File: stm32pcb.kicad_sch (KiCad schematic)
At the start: 11 parts, among them J1 USB_C_Receptacle_USB2.0_16P, J2 Conn_01x04_Pin, J3 USB_C_Receptacle_USB2.0_16P, SW2 SW_Push_DPDT, U1 STM32F103C_8-B_Tx, U2 CH340C, U3 AMS1117-3.3

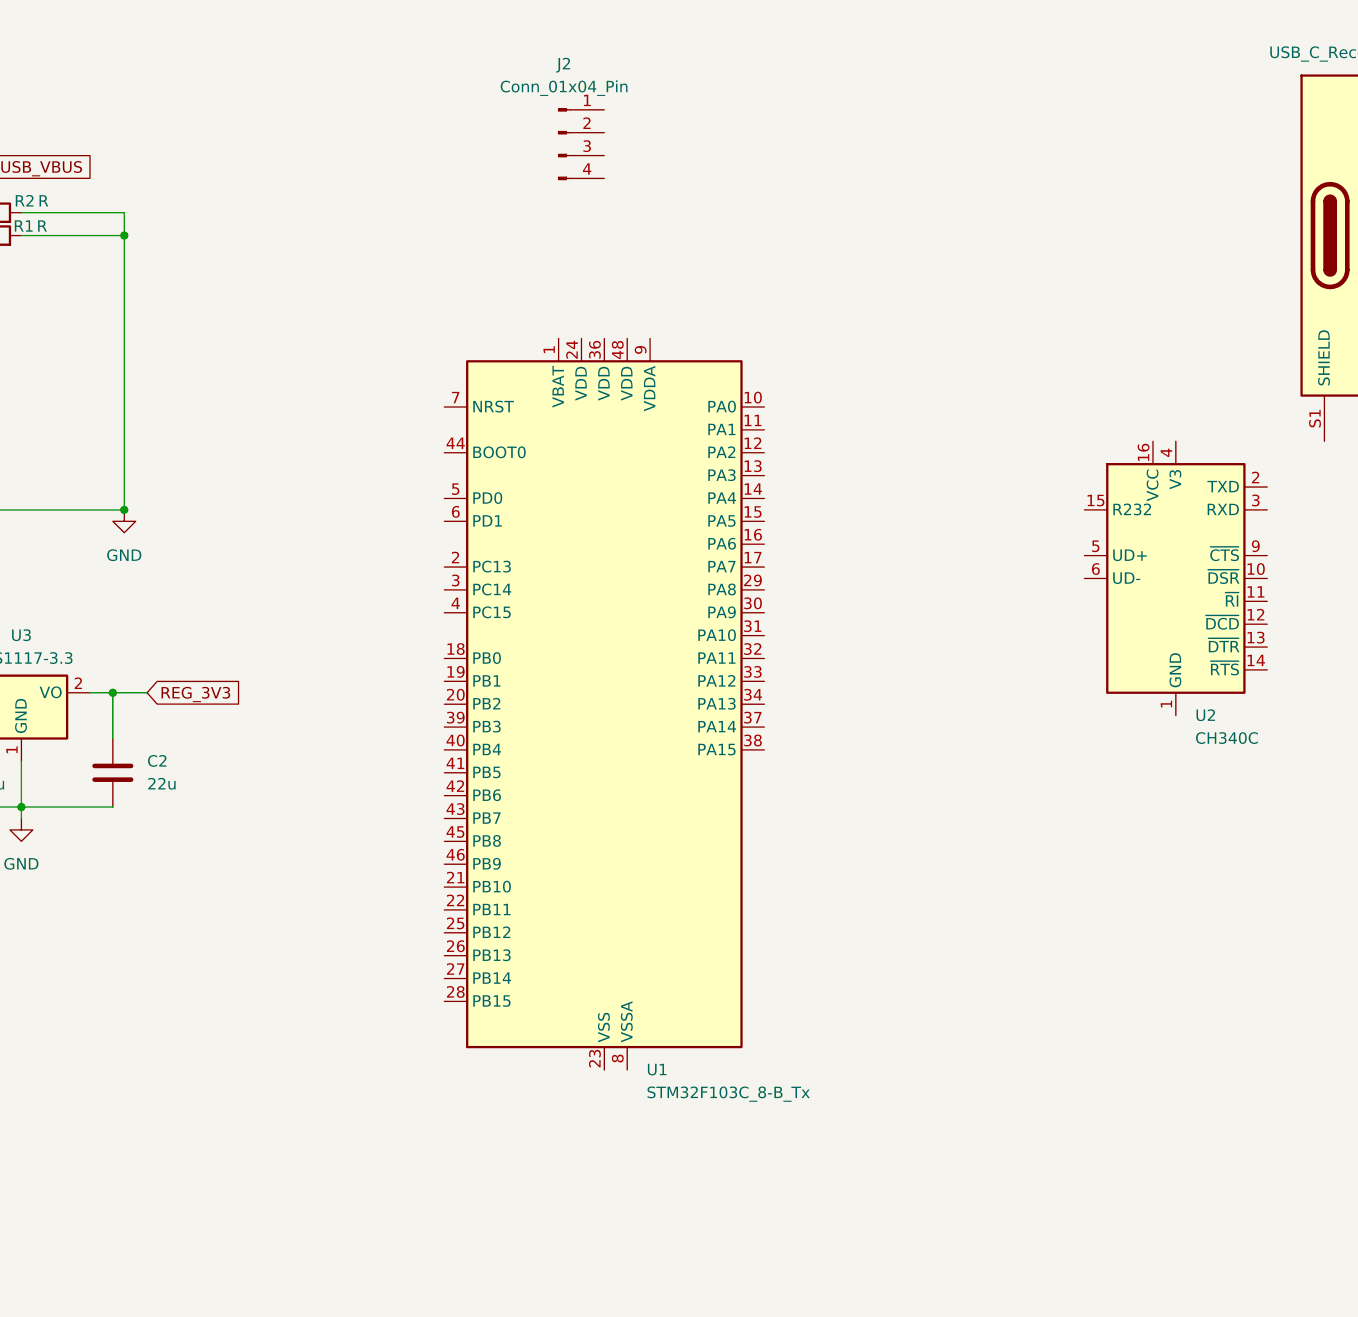
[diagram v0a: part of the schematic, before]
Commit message: 2
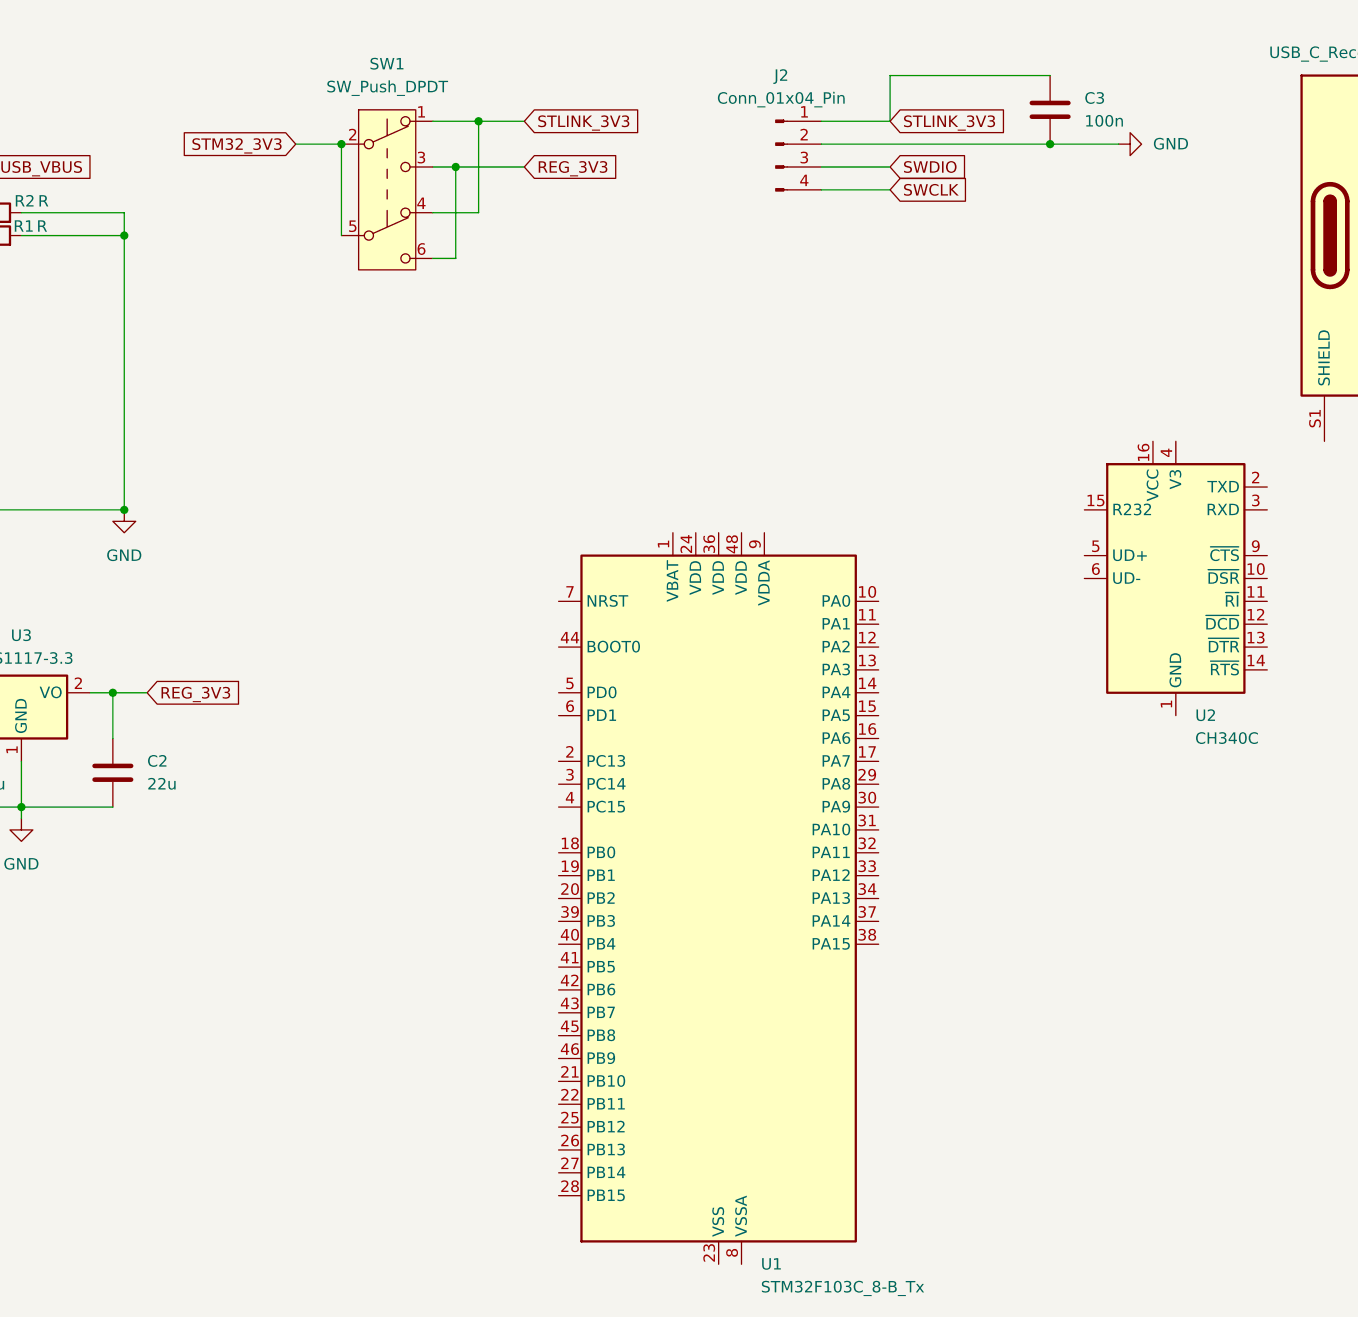
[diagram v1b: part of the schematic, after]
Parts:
- added C3: 100n, Capacitor_SMD:C_0805_2012Metric, symbol Device:C
- added SW1: SW_Push_DPDT, Button_Switch_SMD:SW_DPDT_CK_JS202011JCQN, symbol Switch:SW_Push_DPDT
- C1, C2: footprint (none) -> Capacitor_SMD:C_0805_2012Metric
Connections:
- net GND: now also J2.2 (Pin_2), C3.2
- net REG_3V3: now also SW1.3 (C), SW1.6 (C)
- net STLINK_3V3: now reaches J2.1 (Pin_1)
- net STLINK_3V3: now also C3.1, SW1.1 (A), SW1.4 (A)
- net SWDIO: now reaches J2.3 (Pin_3)
- net SWCLK: now reaches J2.4 (Pin_4)
- new net STM32_3V3: SW1.2 (B), SW1.5 (B)
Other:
- moved on the sheet: J2, U1

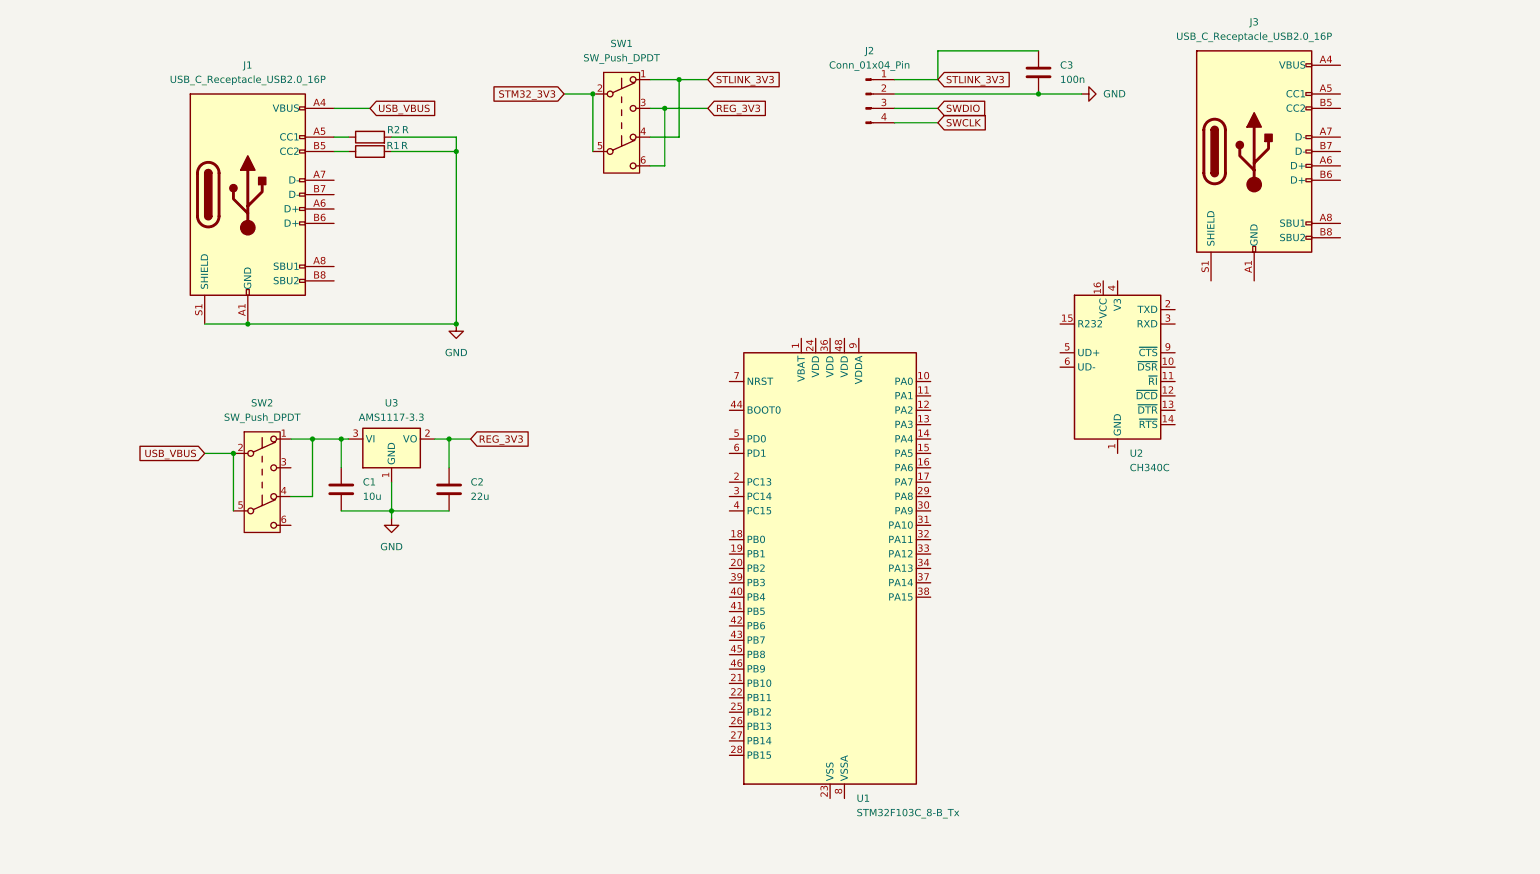
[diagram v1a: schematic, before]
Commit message: update
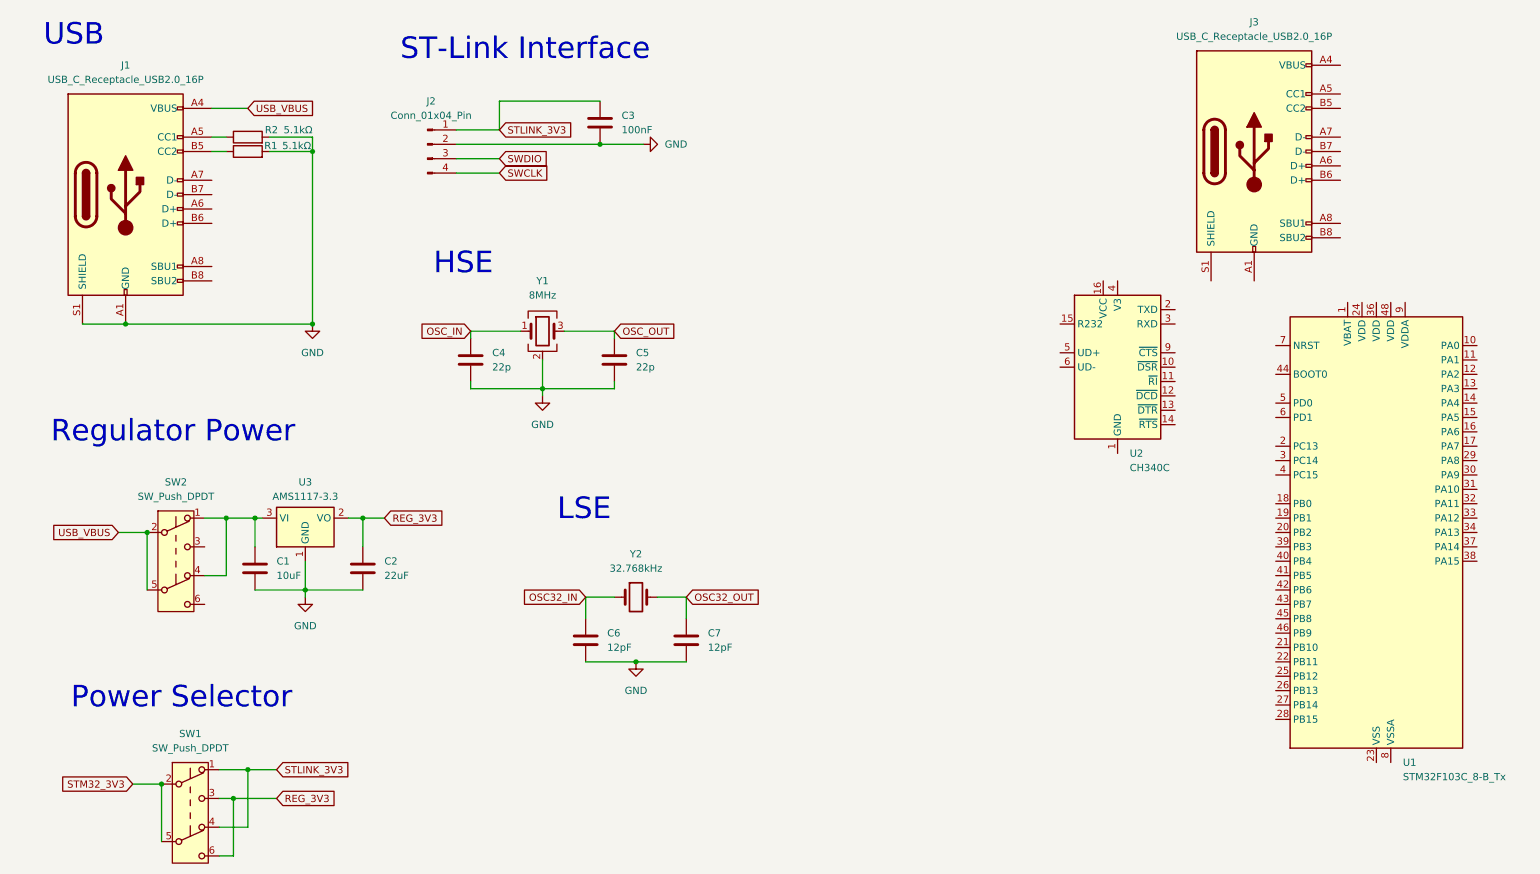
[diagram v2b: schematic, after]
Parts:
- added C4, C5: 22p, Capacitor_SMD:C_0805_2012Metric, symbol Device:C
- added C6, C7: 12pF, Capacitor_SMD:C_0805_2012Metric, symbol Device:C
- added Y1: 8MHz, symbol Device:Crystal_GND24
- added Y2: 32.768kHz, symbol Device:Crystal
- C1: value 10u -> 10uF
- C2: value 22u -> 22uF
- C3: value 100n -> 100nF
- R1, R2: value R -> 5.1kΩ
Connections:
- net GND: now also C4.2, C5.2, C6.2, C7.2, Y1.2 (G), Y1.4 (G)
- new net OSC32_IN: C6.1, Y2.1
- new net OSC32_OUT: C7.1, Y2.2
- new net OSC_IN: C4.1, Y1.1
- new net OSC_OUT: C5.1, Y1.3
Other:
- note added: "HSE"
- note added: "LSE"
- note added: "Power Selector"
- note added: "Regulator Power"
- note added: "ST-Link Interface"
- note added: "USB"
- moved on the sheet: C1, C2, C3, J1, J2, R1, R2, SW1, SW2, U1, U3

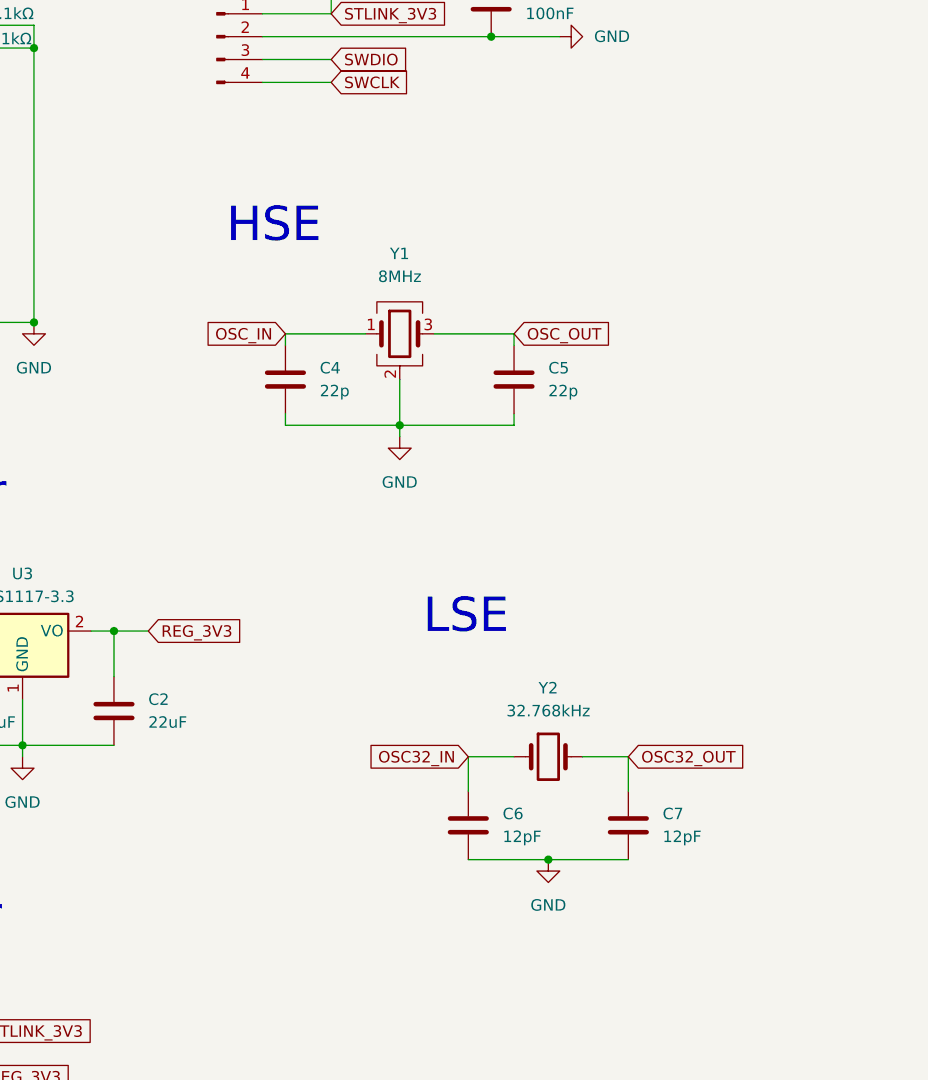
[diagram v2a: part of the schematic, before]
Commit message: update
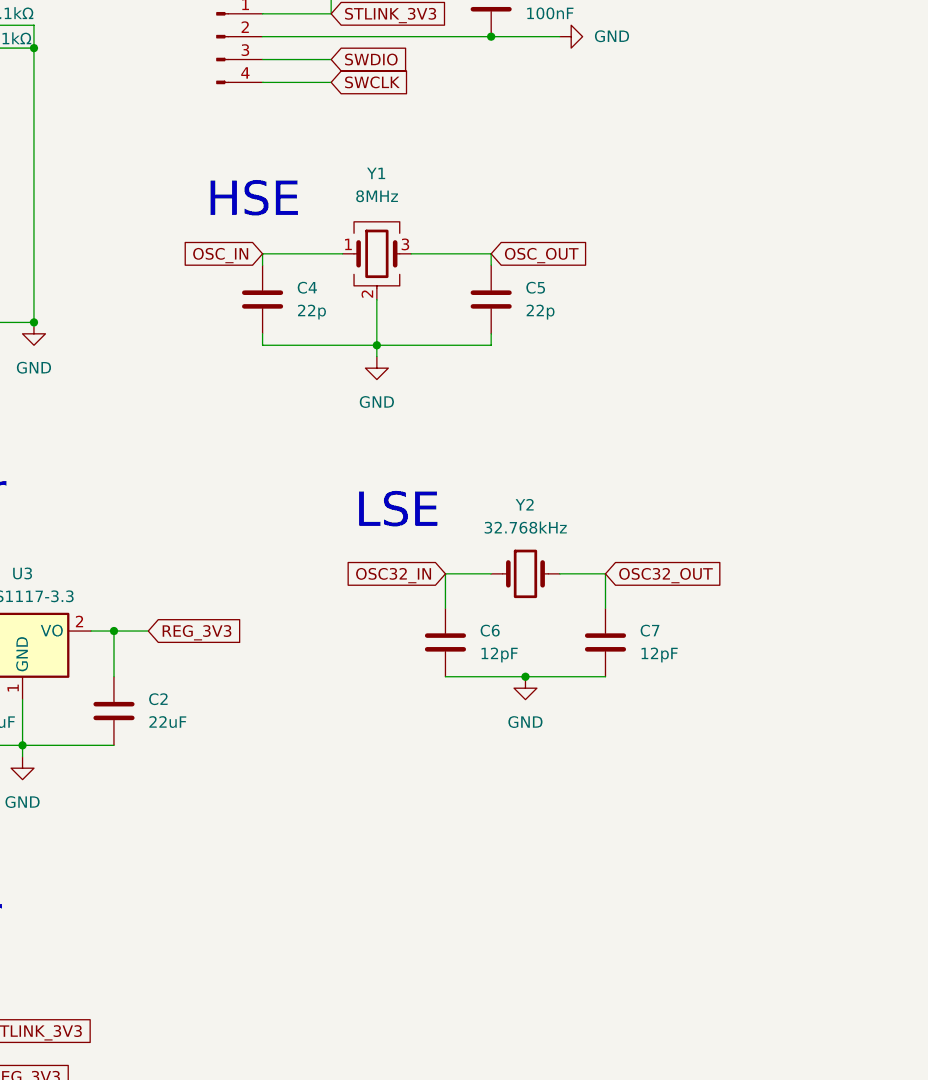
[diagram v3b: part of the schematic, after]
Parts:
- SW1: footprint Button_Switch_SMD:SW_DPDT_CK_JS202011JCQN -> lcsc:SW-SMD_6P-L9.1-W3.5-P2.50
- Y1: footprint (none) -> Crystal:Crystal_SMD_3225-4Pin_3.2x2.5mm
- Y2: footprint (none) -> Crystal:Crystal_SMD_3215-2Pin_3.2x1.5mm
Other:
- moved on the sheet: C4, C5, C6, C7, Y1, Y2

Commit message: update
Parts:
- added C10, C11, C12, C8, C9: 100nF, Capacitor_SMD:C_0805_2012Metric, symbol Device:C
- added D1, D2: LED, symbol Device:LED
- added J4: Conn_01x12_Pin, symbol Connector:Conn_01x12_Pin
- added R3, R4, R7: 10kΩ, Resistor_SMD:R_1206_3216Metric, symbol Device:R
- added R5, R6: 1kΩ, Resistor_SMD:R_1206_3216Metric, symbol Device:R
- added R8: 1.5kΩ, Resistor_SMD:R_1206_3216Metric, symbol Device:R
- added SW3, SW4: SW_Push_DPDT, Button_Switch_SMD:SW_DPDT_CK_JS202011JCQN, symbol Switch:SW_Push_DPDT
- added SW5: TS-1088-AR02016, lcsc:SW-SMD_L3.9-W3.0-P4.45, symbol lcsc:TS-1088-AR02016
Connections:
- net GND: now also U1.23 (VSS), U1.35 (VSS), U1.47 (VSS), U1.8 (VSSA), C10.2, C11.2, C12.2, C8.2, C9.2, D1.1 (K), D2.1 (K), J4.8 (Pin_8), SW3.3 (C), SW3.6 (C), SW4.3 (C), SW4.6 (C), SW5.1
- net REG_3V3: now also R5.2
- net STLINK_3V3: now also R6.2
- net STM32_3V3: now also U1.24 (VDD), U1.36 (VDD), U1.48 (VDD), U1.9 (VDDA), C10.1, C11.1, C8.1, C9.1, J4.9 (Pin_9), R7.2, R8.2, SW3.1 (A), SW3.4 (A), SW4.1 (A), SW4.4 (A)
- net at U1.1 (VBAT): now also J4.1 (Pin_1)
- net at U1.10 (PA0): now also J4.10 (Pin_10)
- net at U1.11 (PA1): now also J4.11 (Pin_11)
- net at U1.12 (PA2): now also J4.12 (Pin_12)
- net at U1.2 (PC13): now also J4.2 (Pin_2)
- net PB2_BOOT1: now reaches U1.20 (PB2)
- net at U1.3 (PC14): now also J4.3 (Pin_3)
- net at U1.4 (PC15): now also J4.4 (Pin_4)
- net BOOT0: now reaches U1.44 (BOOT0)
- net BOOT0: now also R3.1, R4.1
- net at U1.5 (PD0): now also J4.5 (Pin_5)
- net at U1.6 (PD1): now also J4.6 (Pin_6)
- net NRST: now reaches U1.7 (NRST)
- net NRST: now also C12.1, J4.7 (Pin_7), R7.1, SW5.2
- net USB_DP: now reaches J1.A6 (D+)
- net USB_DP: now also J1.B6 (D+), R8.1
- net USB_DN: now reaches J1.A7 (D-)
- net USB_DN: now also J1.B7 (D-)
- new net: D1.2 (A), R5.1
- new net: R3.2, SW3.2 (B), SW3.5 (B)
- new net: R4.2, SW4.2 (B), SW4.5 (B)
- new net: D2.2 (A), R6.1
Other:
- note added: "BOOT"
- note added: "LED"
- note added: "RESET"
- note added: "SoC Power Filter"
- moved on the sheet: C1, C2, C4, C5, C6, C7, J3, SW1, SW2, U1, U2, U3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
